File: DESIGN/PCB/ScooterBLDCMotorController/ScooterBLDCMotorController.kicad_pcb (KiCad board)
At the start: 2 copper layers, 210.3 x 103.4 mm, 30 parts, among them J1 M1 OUTPUT, J10 RC_ENABLE, J2 M1 INPUT, J3 M2 INPUT, J4 M2 OUTPUT, J5 I2C, J6 TEST SWITCH, J7 RC CH 1, J8 RC CH 2, J9 RC_PWR, U1 , U10 , U2 SN74HC14NR, U3 , U4 Teensy4.0, U5 SN74HC14NR, U6 , U7 5V_Voltage_Regulator, U8 3.3V_Voltage_Regulator, U9 

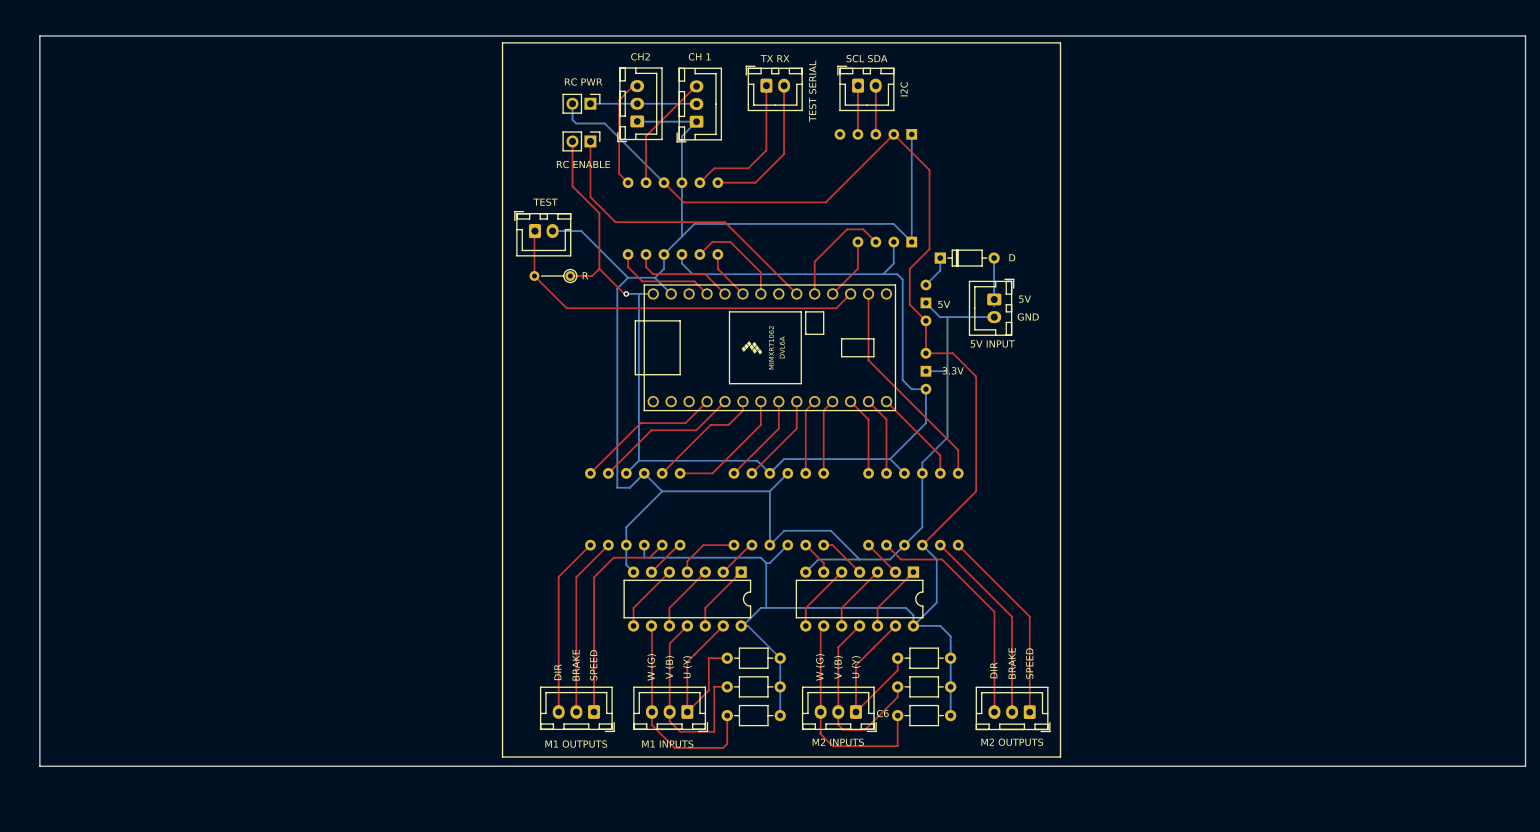
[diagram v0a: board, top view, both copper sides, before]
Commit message: Latest PCB and Rev1.0 release
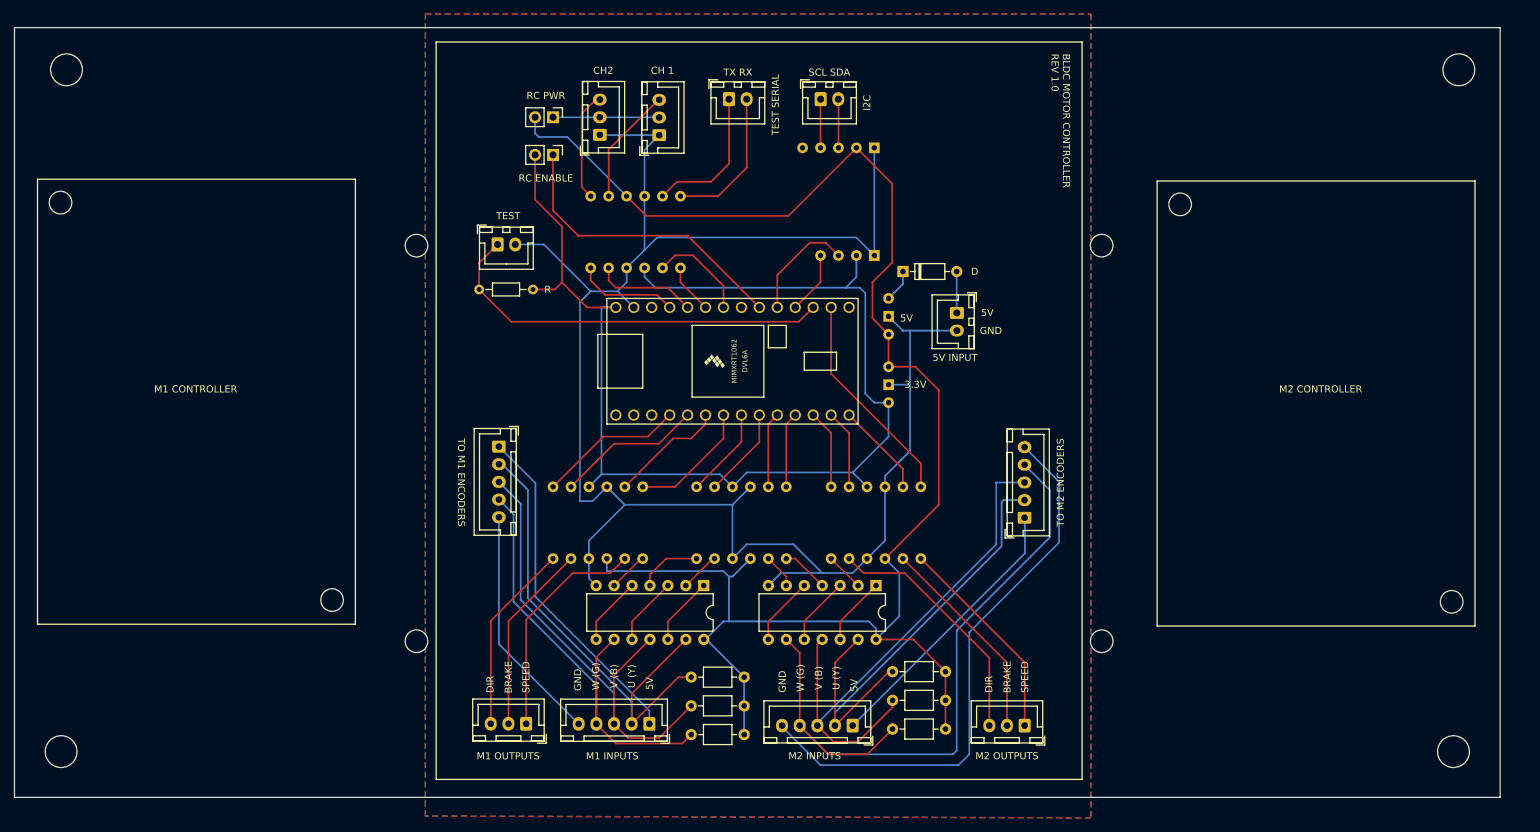
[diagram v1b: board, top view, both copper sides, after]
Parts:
- added J11: TO M2 ENCODER, Connector_JST:JST_XH_B5B-XH-A_1x05_P2.50mm_Vertical, F.Cu at (186.4, 107.1)
- added J12: M2 INPUT, Connector_JST:JST_XH_B5B-XH-A_1x05_P2.50mm_Vertical, F.Cu at (162.1, 136.5)
- added REF**: MountingHole_4.5mm, MountingHole:MountingHole_4.5mm, F.Cu at (247.1, 140.2)
- added REF**: MountingHole_3.2mm_M3, MountingHole:MountingHole_3.2mm_M3, F.Cu at (246.9, 119.0)
- added REF**: MountingHole_3.2mm_M3, MountingHole:MountingHole_3.2mm_M3, F.Cu at (50.0, 62.5)
- added REF**: MountingHole_4.5mm, MountingHole:MountingHole_4.5mm, F.Cu at (247.9, 43.7)
- added REF**: MountingHole_3.2mm_M3, MountingHole:MountingHole_3.2mm_M3, F.Cu at (208.4, 62.7)
- added REF**: MountingHole_3.2mm_M3, MountingHole:MountingHole_3.2mm_M3, F.Cu at (88.4, 118.8)
- added REF**: MountingHole_3.2mm_M3, MountingHole:MountingHole_3.2mm_M3, F.Cu at (197.3, 124.6)
- added REF**: MountingHole_4.5mm, MountingHole:MountingHole_4.5mm, F.Cu at (50.8, 43.7)
- added REF**: MountingHole_3.2mm_M3, MountingHole:MountingHole_3.2mm_M3, F.Cu at (100.3, 68.6)
- added REF**: MountingHole_3.2mm_M3, MountingHole:MountingHole_3.2mm_M3, F.Cu at (197.3, 68.6)
- added REF**: MountingHole_4.5mm, MountingHole:MountingHole_4.5mm, F.Cu at (50.0, 140.2)
- added REF**: MountingHole_3.2mm_M3, MountingHole:MountingHole_3.2mm_M3, F.Cu at (100.3, 124.6)
- J2: value M1 INPUT -> TO M1 ENCODER; footprint Connector_JST:JST_XH_B3B-XH-A_1x03_P2.50mm_Vertical -> Connector_JST:JST_XH_B5B-XH-A_1x05_P2.50mm_Vertical
- J3: value M2 INPUT -> M1 INPUT; footprint Connector_JST:JST_XH_B3B-XH-A_1x03_P2.50mm_Vertical -> Connector_JST:JST_XH_B5B-XH-A_1x05_P2.50mm_Vertical
- R1: footprint Resistor_THT:R_Axial_DIN0204_L3.6mm_D1.6mm_P5.08mm_Vertical -> Resistor_THT:R_Axial_DIN0204_L3.6mm_D1.6mm_P7.62mm_Horizontal
- moved J2 46.1 mm to (112.0, 97.0), turned to -90 degrees
- moved J3 29.3 mm to (133.3, 136.3)
- moved J1 9.76 mm to (115.9, 136.3)
- moved C1 5.76 mm to (139.2, 129.7)
- moved C2 5.76 mm to (139.2, 133.7)
- moved C3 5.76 mm to (139.2, 137.8)
- moved J5 5.63 mm to (157.6, 47.8)
- moved J6 5.63 mm to (111.8, 68.4)
- moved J7 5.63 mm to (134.7, 52.9)
- moved U10 5.63 mm to (127.5, 66.7)
- moved U2 5.63 mm to (141.0, 116.7)
- moved U3 5.63 mm to (150.2, 107.8)
- moved U5 5.63 mm to (165.4, 116.7)
- moved U7 5.63 mm to (167.2, 78.6)
- moved U8 5.63 mm to (167.2, 88.3)
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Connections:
- J2 pad 1: /M1 Y -> Net-(J2-Pad1)
- J2 pad 2: /M1 B -> /M1 Y
- J2 pad 3: /M1 G -> /M1 B
- J3 pad 1: /M2 Y -> Net-(J2-Pad1)
- J3 pad 2: /M2 B -> /M1 Y
- J3 pad 3: /M2 G -> /M1 B
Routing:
- net Net-(J11-Pad5): track 0.00 -> 80.2 mm
- net /M2 G: track 31.5 -> 100.9 mm
- net /M2 B: track 27.3 -> 75.7 mm
- net Net-(J2-Pad1): track 0.00 -> 48.1 mm
- net /M1 Y: track 25.8 -> 70.7 mm
- net /M2 Y: track 24.6 -> 69.1 mm
- net Net-(J11-Pad1): track 0.00 -> 39.5 mm
- net /M1 B: track 29.6 -> 68.7 mm
- net /M1 G: track 30.3 -> 65.6 mm
- net Net-(J2-Pad5): track 0.00 -> 33.9 mm
- net Net-(J6-Pad1): track 53.9 -> 57.5 mm
- net /3v: track 168.1 -> 170.1 mm, vias 1 -> 0
- net /M2 SPEED: track 27.8 -> 29.7 mm
- net /M2 BRAKE: track 27.8 -> 29.7 mm
- net /M2 DIR: track 33.4 -> 35.3 mm
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- added copper zone on B.Cu, net /GND
- added copper zone on F.Cu, net /GND
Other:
- board size 210.3 x 103.4 mm -> 210.3 x 109 mm
- board text added: "BLDC MOTOR CONTROLLER REV 1.0"
- board text added: "M1 CONTROLLER"
- board text added: "M2 CONTROLLER"
- board text added: "TO M1 ENCODERS"
- board text added: "TO M2 ENCODERS"
